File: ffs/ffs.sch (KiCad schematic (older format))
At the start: 34 parts, among them J1 EURO_PWR_2x5, J2 Conn_01x10_Male, U1 4015, U10 4051, U12 4017, U13 4017, U2 4051, U3 4051, U4 4046, U5 4081, U6 4017, U7 4017, U8 4015, U9 4051

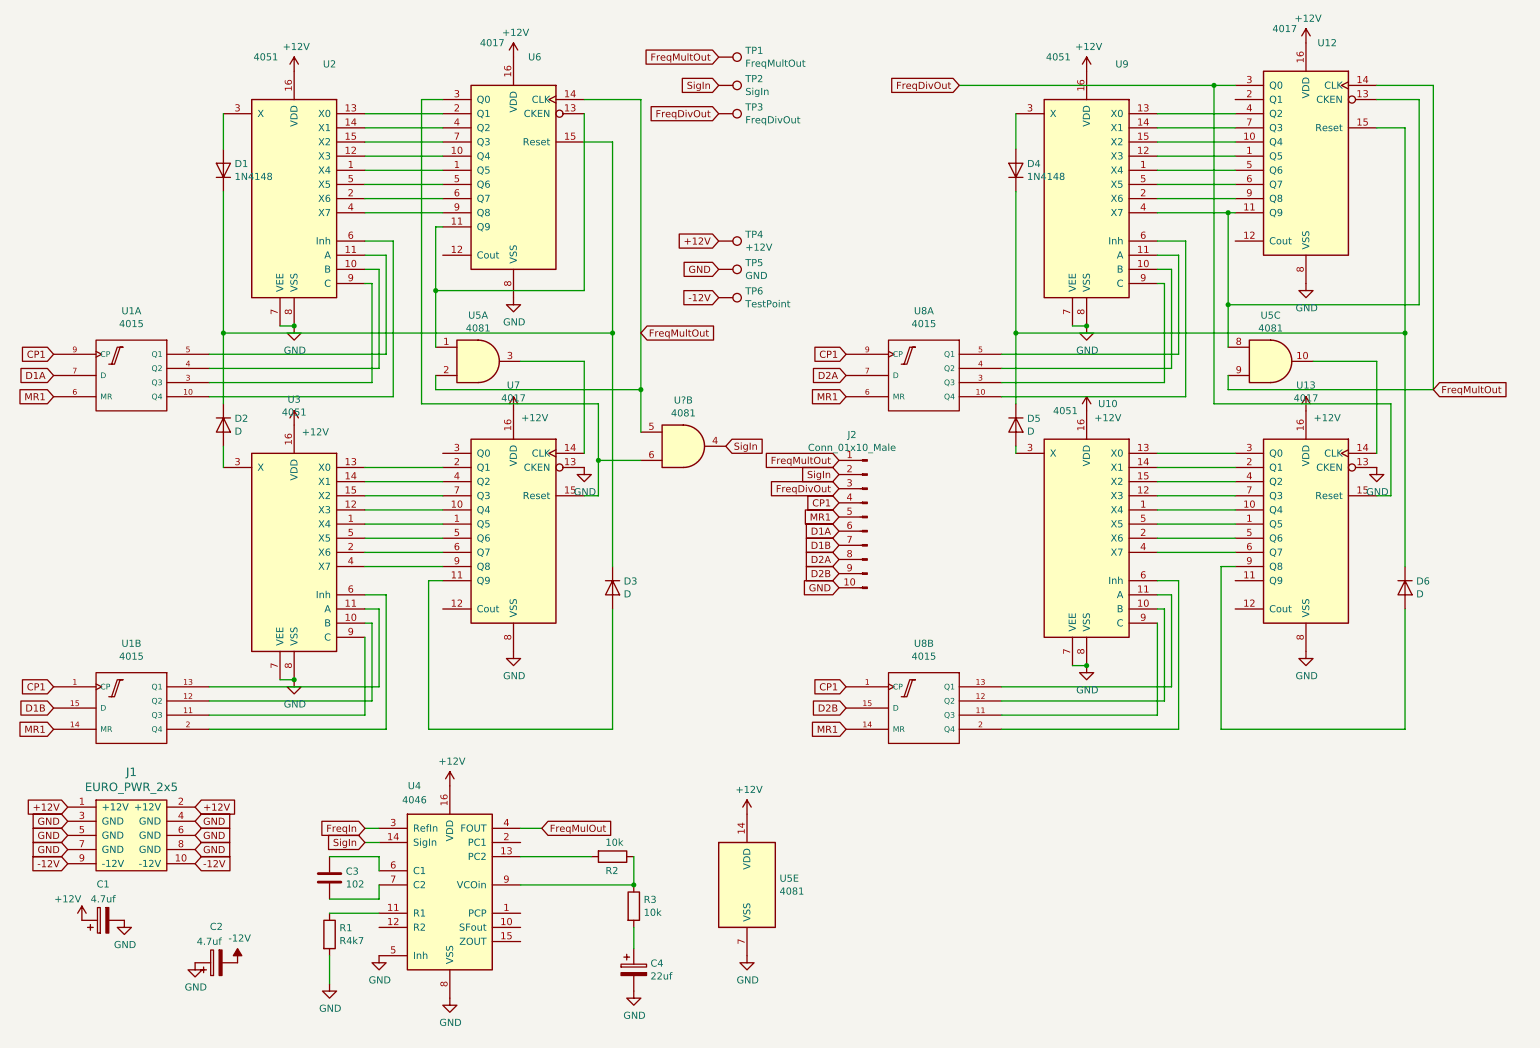
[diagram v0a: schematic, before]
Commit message: ffs routing done
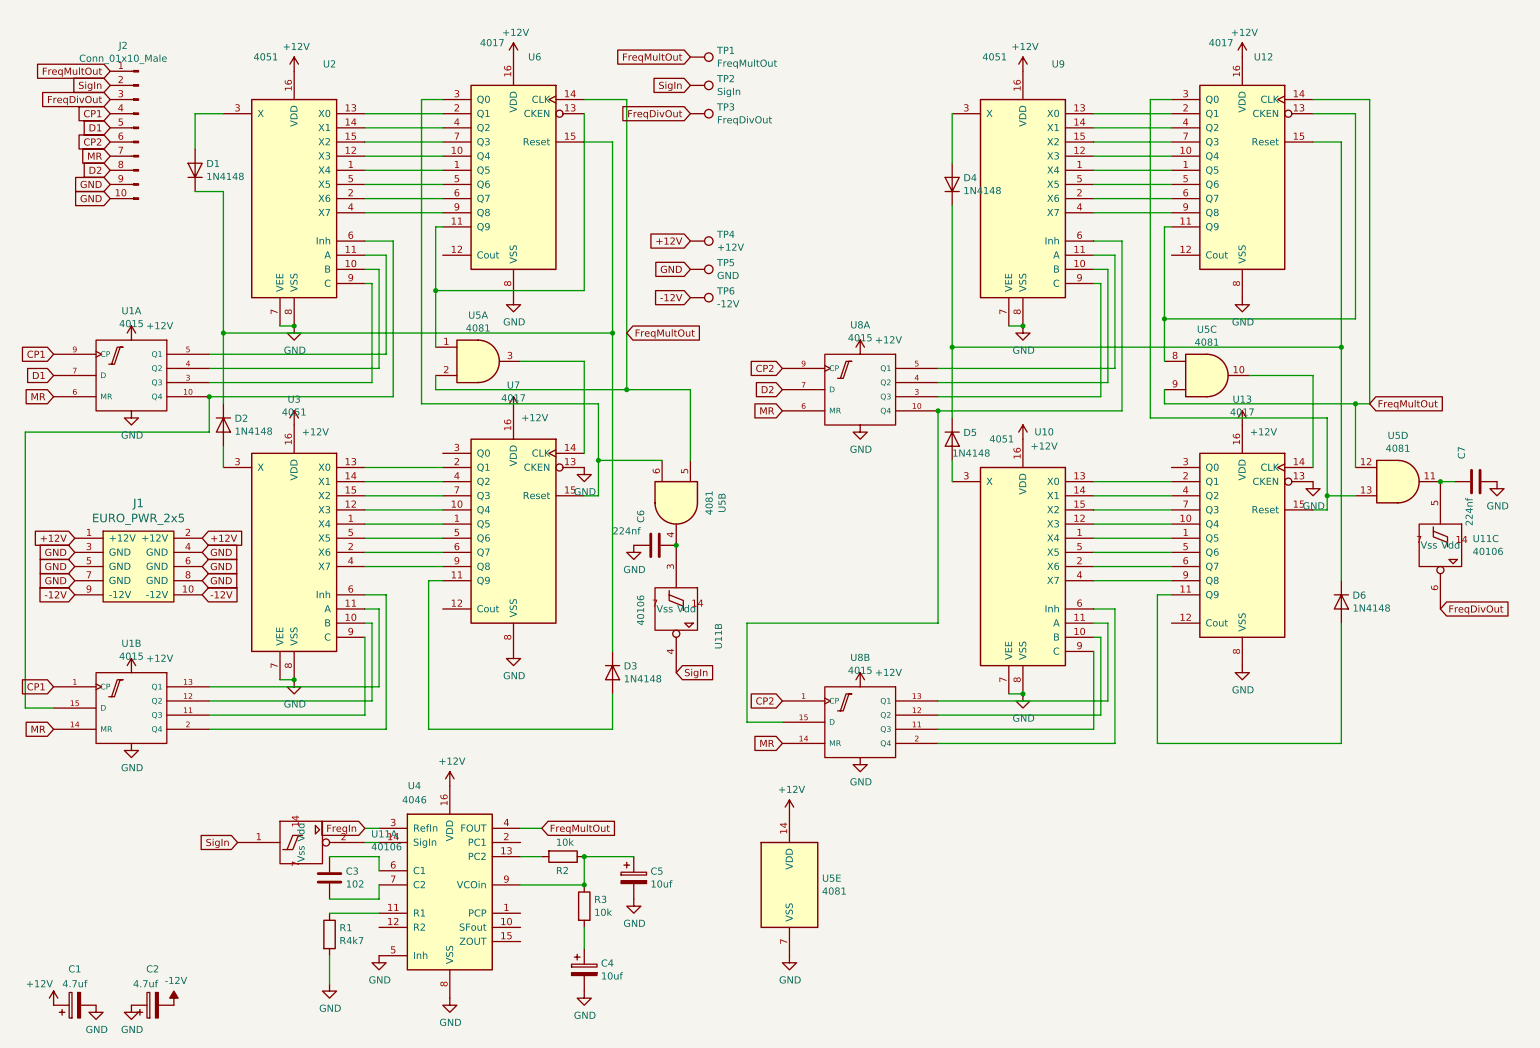
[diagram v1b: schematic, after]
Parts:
- added C5: 10uf, Capacitor_THT:CP_Radial_D8.0mm_P2.50mm, symbol Device:CP
- added C6, C7: 224nf, Capacitor_THT:C_Disc_D4.3mm_W1.9mm_P5.00mm, symbol Device:C
- added U11: 40106, Package_DIP:DIP-16_W7.62mm_Socket, symbol 4xxx_IEEE:40106
- added unit 4 of U5
- C4: value 22uf -> 10uf
- D2, D3, D5, D6: value D -> 1N4148
- TP6: value TestPoint -> -12V
- U5: renamed from U?; footprint (none) -> Package_DIP:DIP-14_W7.62mm_Socket
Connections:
- net FreqMulOut is gone; now on net FreqMultOut: U4.4 (FOUT)
- net Vdd is gone; now on net +12V: U1.16 (Vdd), U1.16 (Vdd), U8.16 (Vdd), U8.16 (Vdd)
- net Vss is gone; now on net GND: U1.8 (Vss), U1.8 (Vss), U8.8 (Vss), U8.8 (Vss)
- net CP1: no longer U8.1 (CP), U8.9 (CP)
- net FreqDivOut: now also U11.6; no longer U12.3 (Q0), U13.15 (Reset)
- net FreqMultOut: now also U5.12
- net GND: now also J2.9 (Pin_9), C5.2, C6.2, C7.1
- net SigIn: now also U11.1, U11.4; no longer U4.14 (SigIn), U5.4
- net at U1.10 (Q4), U2.6 (Inh): now also U1.15 (D)
- net at R2.1, R3.1, U4.9 (VCOin): now also C5.1
- net at U12.1 (Q5): now also U9.1 (X4); no longer U9.12 (X3)
- net at U12.10 (Q4): now also U9.12 (X3); no longer U9.15 (X2)
- net at U12.11 (Q9), U12.13 (CKEN), U5.8: no longer U9.4 (X7)
- net at U12.2 (Q1): now also U9.13 (X0)
- net at U12.4 (Q2): now also U9.14 (X1); no longer U9.13 (X0)
- net at U12.5 (Q6): now also U9.5 (X5); no longer U9.1 (X4)
- net at U12.6 (Q7): now also U9.2 (X6); no longer U9.5 (X5)
- net at U12.7 (Q3): now also U9.15 (X2); no longer U9.14 (X1)
- net at U12.9 (Q8): now also U9.4 (X7); no longer U9.2 (X6)
- net at U8.10 (Q4), U9.6 (Inh): now also U8.15 (D)
- net at U13.1 (Q5): now also U10.1 (X4); no longer U10.5 (X5)
- net at U13.10 (Q4): now also U10.12 (X3); no longer U10.1 (X4)
- net at U13.11 (Q9): now also D6.2 (A)
- net at U13.2 (Q1): now also U10.13 (X0); no longer U10.14 (X1)
- net at U13.3 (Q0): no longer U10.13 (X0)
- net at U13.4 (Q2): now also U10.14 (X1); no longer U10.15 (X2)
- net at U13.5 (Q6): now also U10.5 (X5); no longer U10.2 (X6)
- net at U13.6 (Q7): now also U10.2 (X6); no longer U10.4 (X7)
- net at U13.7 (Q3): now also U10.15 (X2); no longer U10.12 (X3)
- net at U13.9 (Q8): now also U10.4 (X7); no longer D6.2 (A)
- net D1A renamed CP2
- net CP2: now also U8.1 (CP), U8.9 (CP); no longer U1.7 (D)
- net D1B renamed MR
- net MR: now also U1.14 (MR), U1.6 (MR), U8.14 (MR), U8.6 (MR); no longer U1.15 (D)
- net D2A renamed D2
- removed net D2B: J2.9 (Pin_9), U8.15 (D)
- removed net MR1: J2.5 (Pin_5), U1.14 (MR), U1.6 (MR), U8.14 (MR), U8.6 (MR)
- new net: C6.1, U11.3, U5.4
- new net: C7.2, U11.5, U5.11
- new net: U11.2, U4.14 (SigIn)
- new net: U12.3 (Q0), U13.15 (Reset), U5.13
- new net D1: J2.5 (Pin_5), U1.7 (D)
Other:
- moved on the sheet: C1, C2, C4, D1, D3, D4, D5, D6, J1, J2, R2, R3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
